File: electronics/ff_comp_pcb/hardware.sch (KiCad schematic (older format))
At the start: 34 parts, among them J3 Conn_01x07_Female, U2 A33

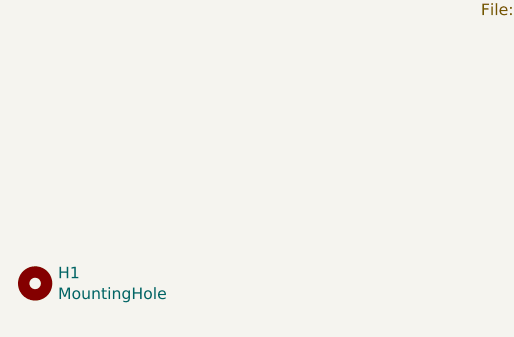
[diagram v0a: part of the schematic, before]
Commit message: Added gerbers for R0.1 comp pcb.
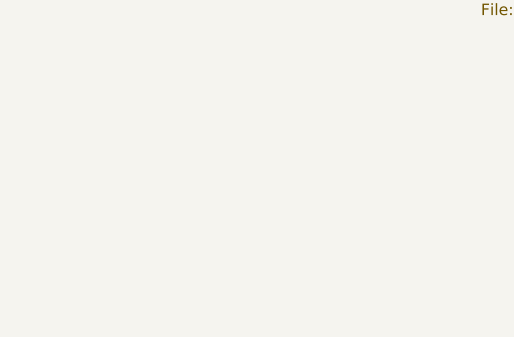
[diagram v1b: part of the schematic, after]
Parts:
- removed H1: MountingHole, MountingHole:MountingHole_3.2mm_M3, symbol Mechanical:MountingHole
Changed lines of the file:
@@
 	6500 5600 6450 5600
-$Comp
-L Mechanical:MountingHole H1
-U 1 1 61489B61
-P 700 7550
-F 0 "H1" H 800 7596 50  0000 L CNN
-F 1 "MountingHole" H 800 7505 50  0000 L CNN
-F 2 "MountingHole:MountingHole_3.2mm_M3" H 700 7550 50  0001 C CNN
-F 3 "~" H 700 7550 50  0001 C CNN
-	1    700  7550
-	1    0    0    -1
-$EndComp
 $Comp
 L Connector:Conn_01x07_Female J3
